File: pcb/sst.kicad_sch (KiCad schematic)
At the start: 36 parts, among them X1 CONN_INPUTS, X2 CONN_PWR, X3 CONN_SPI, X4 CONN_I2C, X5 CONN_INPUTS

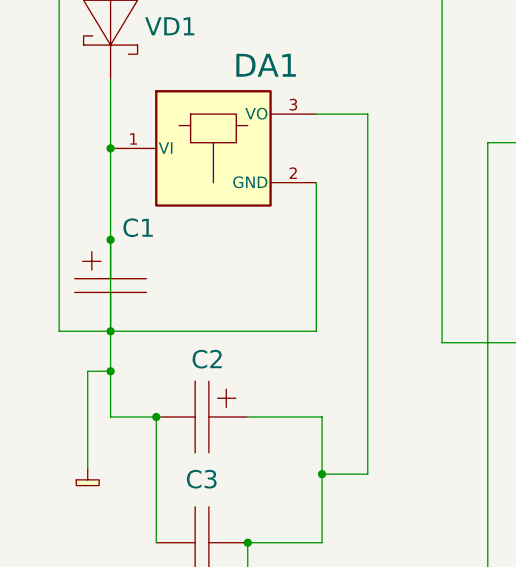
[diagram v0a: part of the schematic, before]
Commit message: [2024-12-24 15:48] coursework for this day
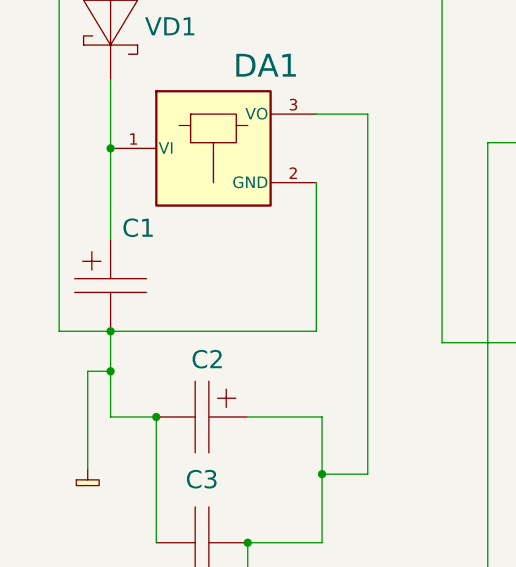
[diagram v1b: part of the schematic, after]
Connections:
- net GND: no longer C1.1, DA1.1 (VI), VD1.1 (K)
- new net: C1.1, DA1.1 (VI), VD1.1 (K)
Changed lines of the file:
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@@
-	)
-	(junction
-		(at 31.75 214.63)
-		(diameter 0)
-		(color 0 0 0 0)
 	)
 	(junction
@@
 		)
 		(stroke
-			(width 0)
-			(type default)
-		)
-	)
-	(wire
-		(pts
-			(xy 31.75 224.79) (xy 31.75 214.63)
-		)
-		(stroke
